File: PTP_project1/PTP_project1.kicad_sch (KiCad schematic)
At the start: 2 parts

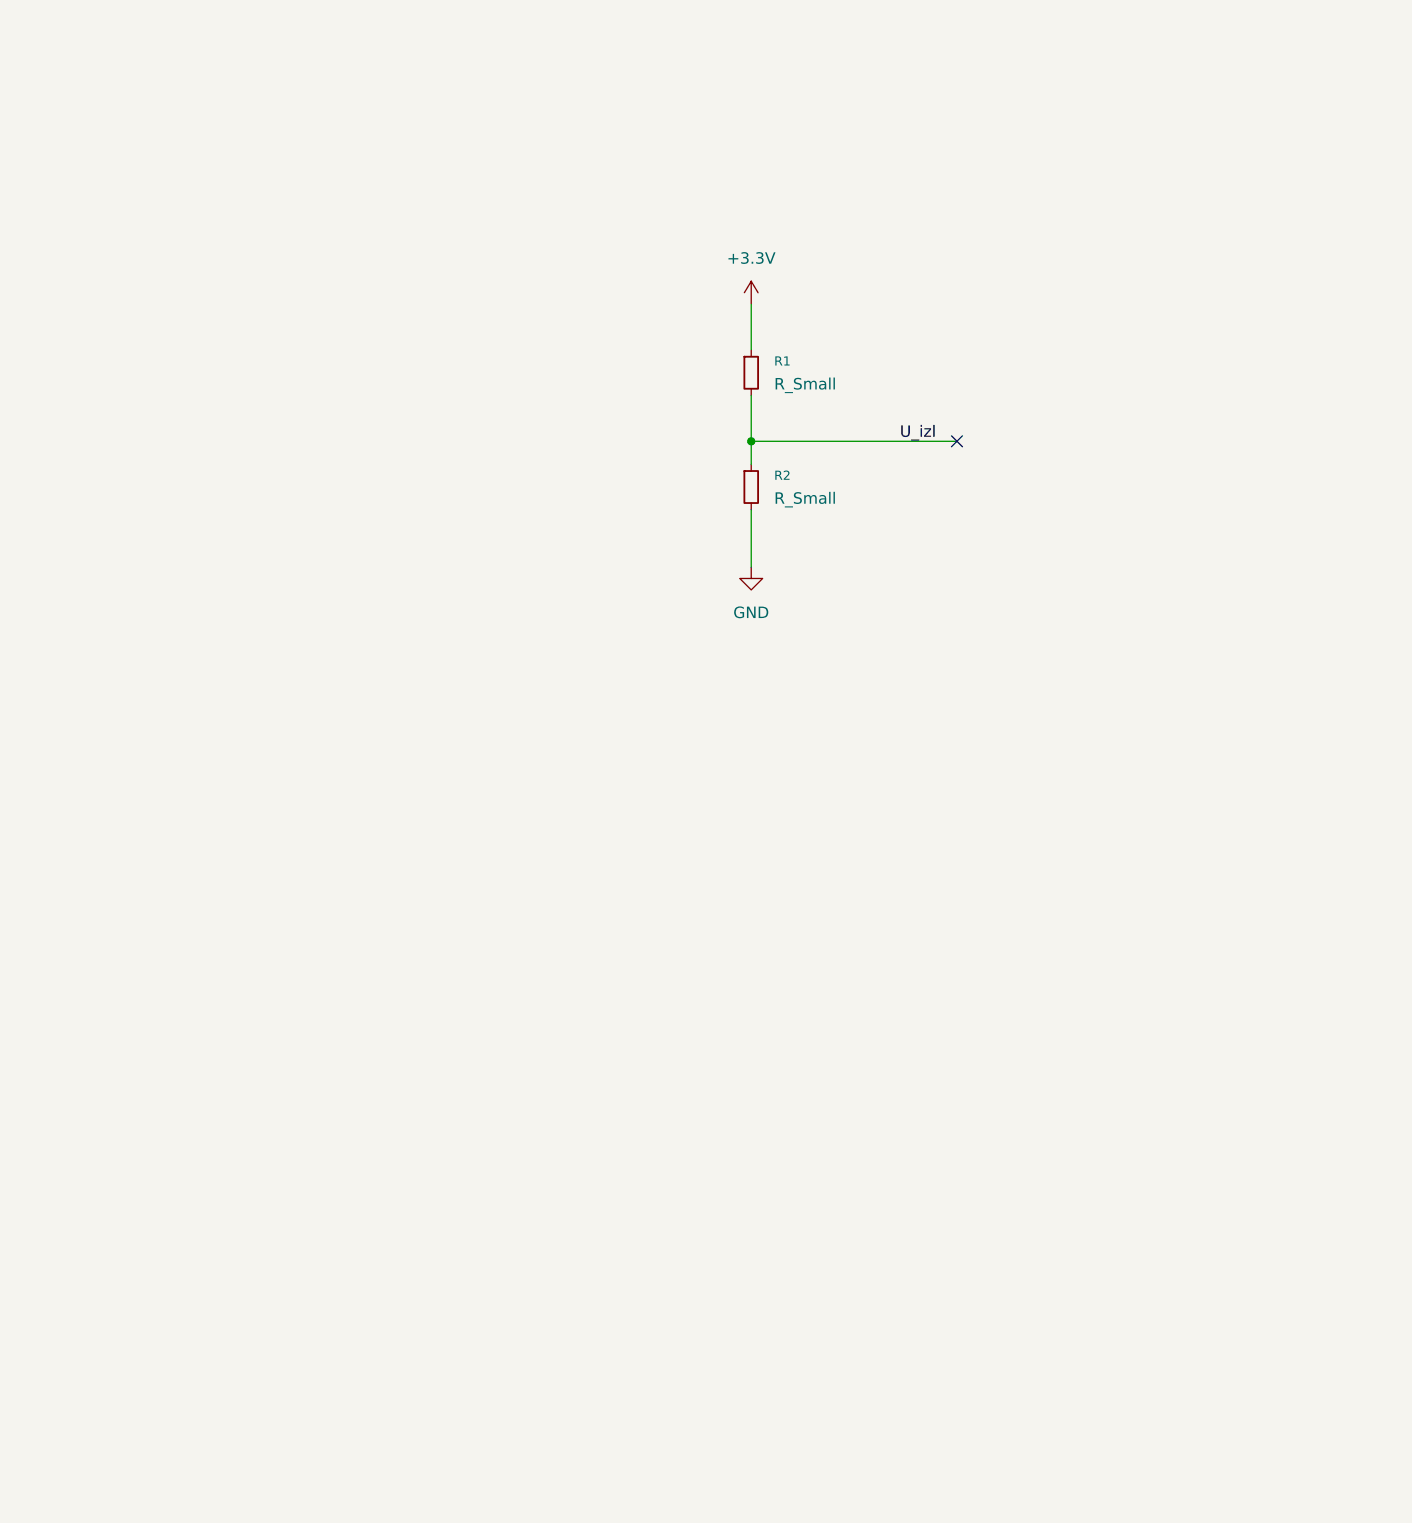
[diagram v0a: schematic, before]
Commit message: LV_2
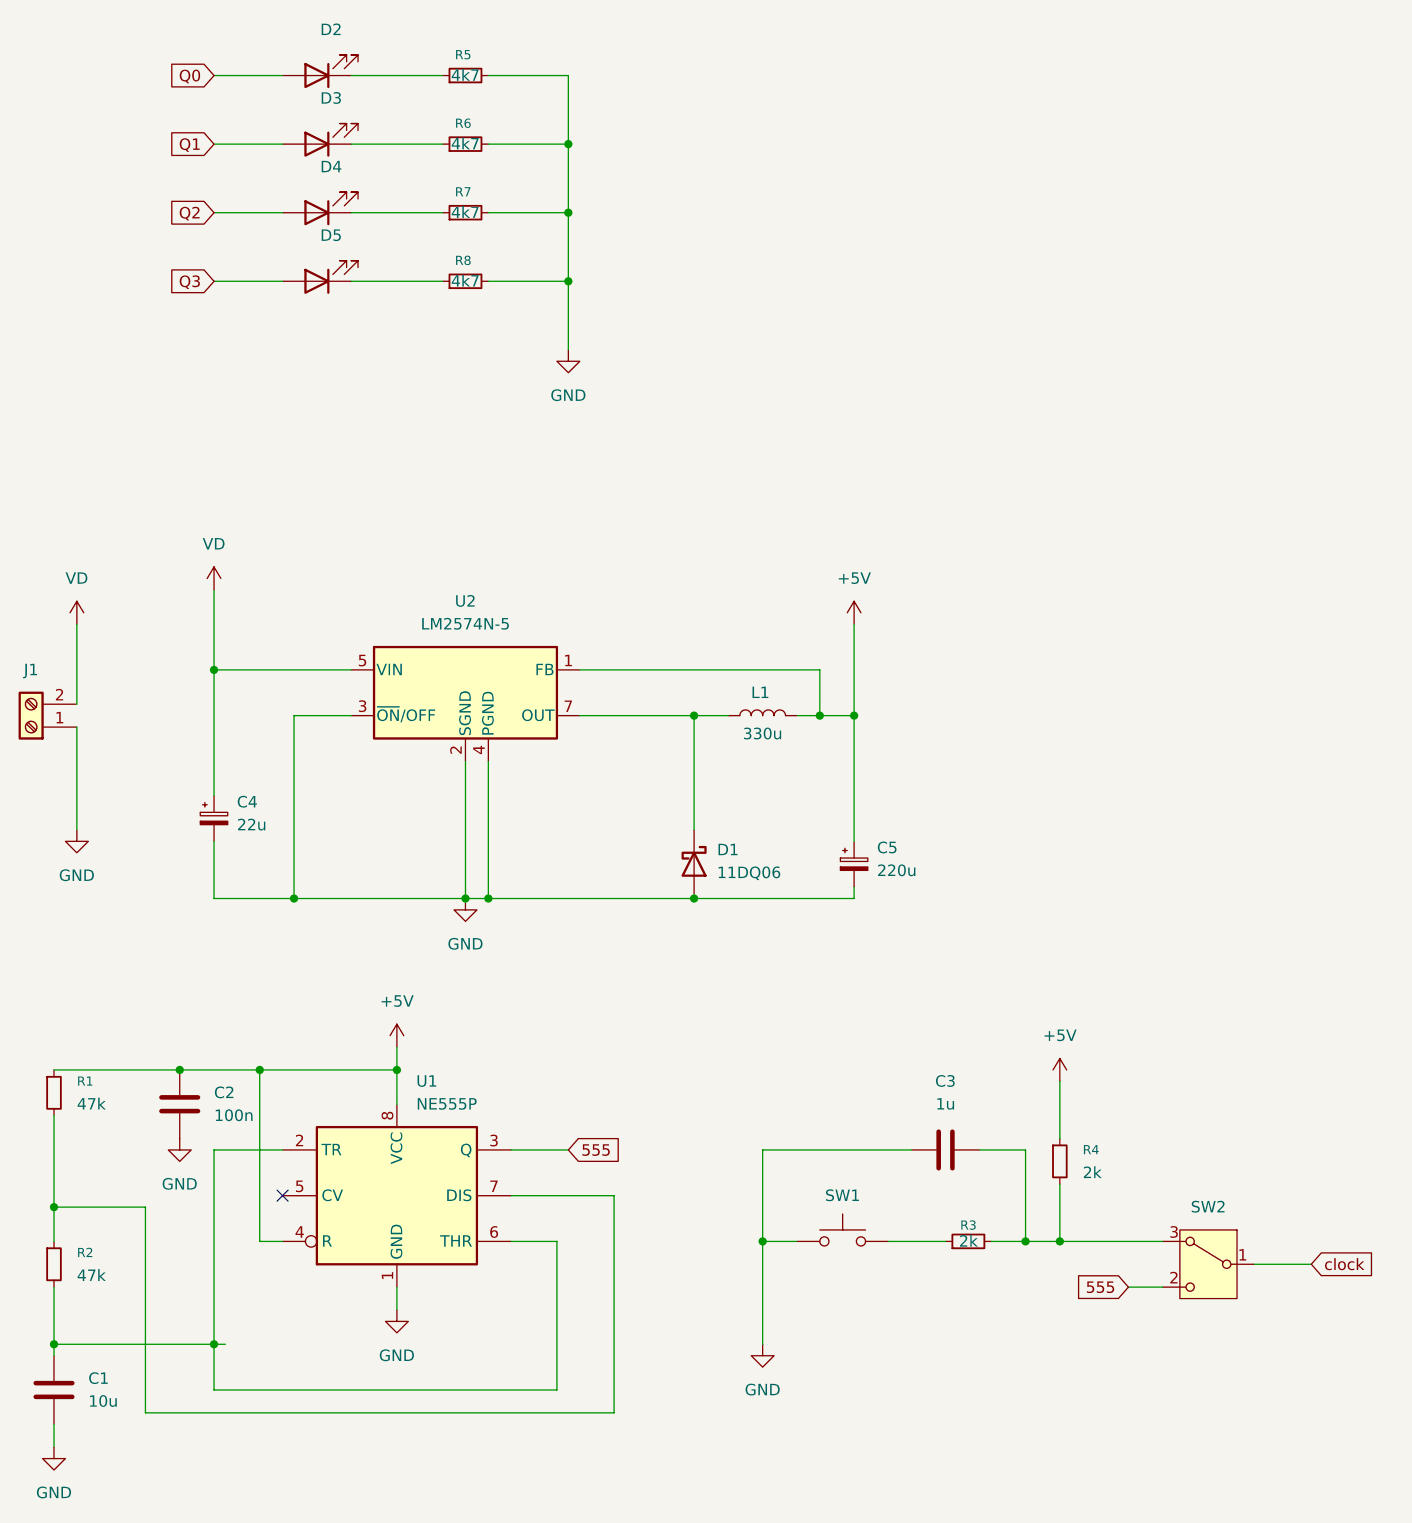
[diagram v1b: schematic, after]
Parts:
- added C1: 10u, symbol Device:C
- added C2: 100n, symbol Device:C
- added C3: 1u, symbol Device:C
- added C4: 22u, symbol Device:C_Polarized_Small
- added C5: 220u, symbol Device:C_Polarized_Small
- added D1: 11DQ06, Diode_SMD:D_SMA, symbol Diode:SS310
- added D2, D3, D4, D5: LED, symbol Device:LED
- added J1: Screw_Terminal_01x02, symbol Connector:Screw_Terminal_01x02
- added L1: 330u, symbol Device:L
- added R3, R4: 2k, symbol Device:R_Small
- added R5, R6, R7, R8: 4k7, symbol Device:R_Small
- added SW1: ~, symbol Switch:SW_MEC_5G
- added SW2: SW_SPDT_312, symbol Switch:SW_SPDT_312
- added U1: NE555P, Package_DIP:DIP-8_W7.62mm, symbol Timer:NE555P
- added U2: LM2574N-5, Package_DIP:DIP-8_W7.62mm, symbol Regulator_Switching:LM2574N-5
- R1, R2: value R_Small -> 47k
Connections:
- net GND: now also C1.2, C2.2, C3.1, C4.2, C5.2, D1.2 (A), J1.1 (Pin_1), R5.2, R6.2, R7.2, R8.2, SW1.1 (A), SW1.2 (A), U1.1 (GND), U2.2 (SGND), U2.3 (~{ON}/OFF), U2.4 (PGND); no longer R2.2
- net +3.3V renamed +5V
- net +5V: now also C2.1, C5.1, L1.2, R4.1, U1.4 (R), U1.8 (VCC), U2.1 (FB)
- net U_izl: no longer names the net of R1.2, R2.1
- net U_izl: now also U1.7 (DIS)
- new net: D2.1 (K), R5.1
- new net: D1.1 (K), L1.1, U2.7 (OUT)
- new net: D5.1 (K), R8.1
- new net: C1.1, R2.2, U1.2 (TR), U1.6 (THR)
- new net: D4.1 (K), R7.1
- new net: C3.2, R3.2, R4.2, SW2.3 (A)
- new net: R3.1, SW1.3 (B), SW1.4 (B)
- new net: D3.1 (K), R6.1
- new net 555: SW2.2 (C), U1.3 (Q)
- new net Q0: D2.2 (A)
- new net Q1: D3.2 (A)
- new net Q2: D4.2 (A)
- new net Q3: D5.2 (A)
- new net VD: C4.1, J1.2 (Pin_2), U2.5 (VIN)
- new net clock: SW2.1 (B)
